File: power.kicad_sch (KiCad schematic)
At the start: 10 parts, among them U1 NCP1117-3.3_SOT223, U15 NCP1117-5.0_SOT223

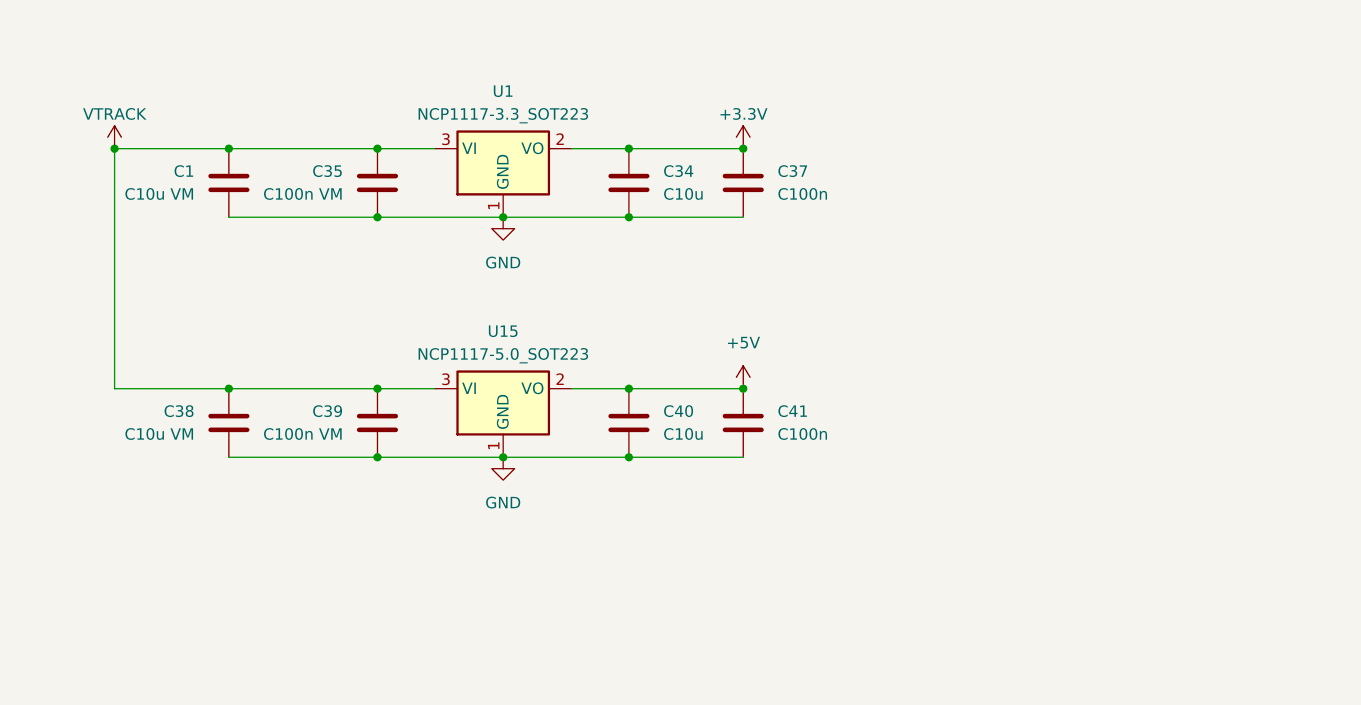
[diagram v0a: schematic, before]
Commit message: Add new routing strategy
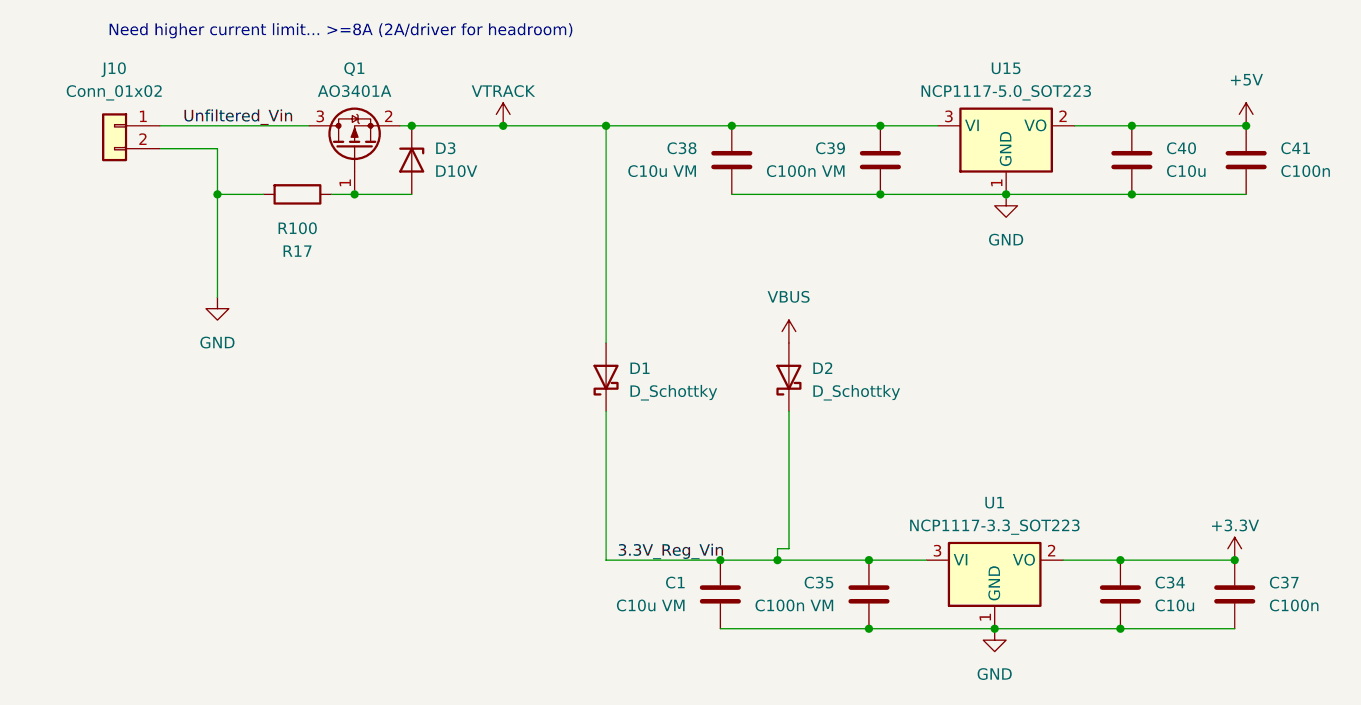
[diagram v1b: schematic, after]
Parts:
- added D1, D2: D_Schottky, Diode_SMD:D_SMA_Handsoldering, symbol Device:D_Schottky
- added D3: D10V, Diode_SMD:D_SOD-323_HandSoldering, symbol Device:D_Zener
- added J10: Conn_01x02, Connector_Phoenix_MC:PhoenixContact_MCV_1,5_2-G-3.5_1x02_P3.50mm_Vertical, symbol Connector_Generic:Conn_01x02
- added Q1: AO3401A, Package_TO_SOT_SMD:SOT-23, symbol Transistor_FET:AO3401A
- added R17: R100, Resistor_SMD:R_0402_1005Metric, symbol Device:R
- C1, C34, C38, C40: footprint (none) -> Capacitor_SMD:C_1206_3216Metric_Pad1.33x1.80mm_HandSolder
- C35, C37, C39, C41: footprint (none) -> Capacitor_SMD:C_0805_2012Metric_Pad1.18x1.45mm_HandSolder
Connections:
- net GND: now also J10.2 (Pin_2), R17.2
- net VTRACK: now also D1.2 (A), D3.1 (K), Q1.2 (S); no longer C1.1, C35.1, U1.3 (VI)
- new net: D3.2 (A), Q1.1 (G), R17.1
- new net 3.3V_Reg_Vin: C1.1, C35.1, D1.1 (K), D2.1 (K), U1.3 (VI)
- new net Unfiltered_Vin: J10.1 (Pin_1), Q1.3 (D)
- new net VBUS: D2.2 (A)
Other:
- note added: "Need higher current limit... >=8A (2A/driver for headroom)"
- moved on the sheet: C1, C34, C35, C37, C38, C39, C40, C41, U1, U15
